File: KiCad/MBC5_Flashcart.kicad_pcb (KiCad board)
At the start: 2 copper layers, 51.1 x 61.3 mm, 10 parts, among them J0 CartBus, U1 MBC5, U2 MBM29F033C, U3 FM18W08

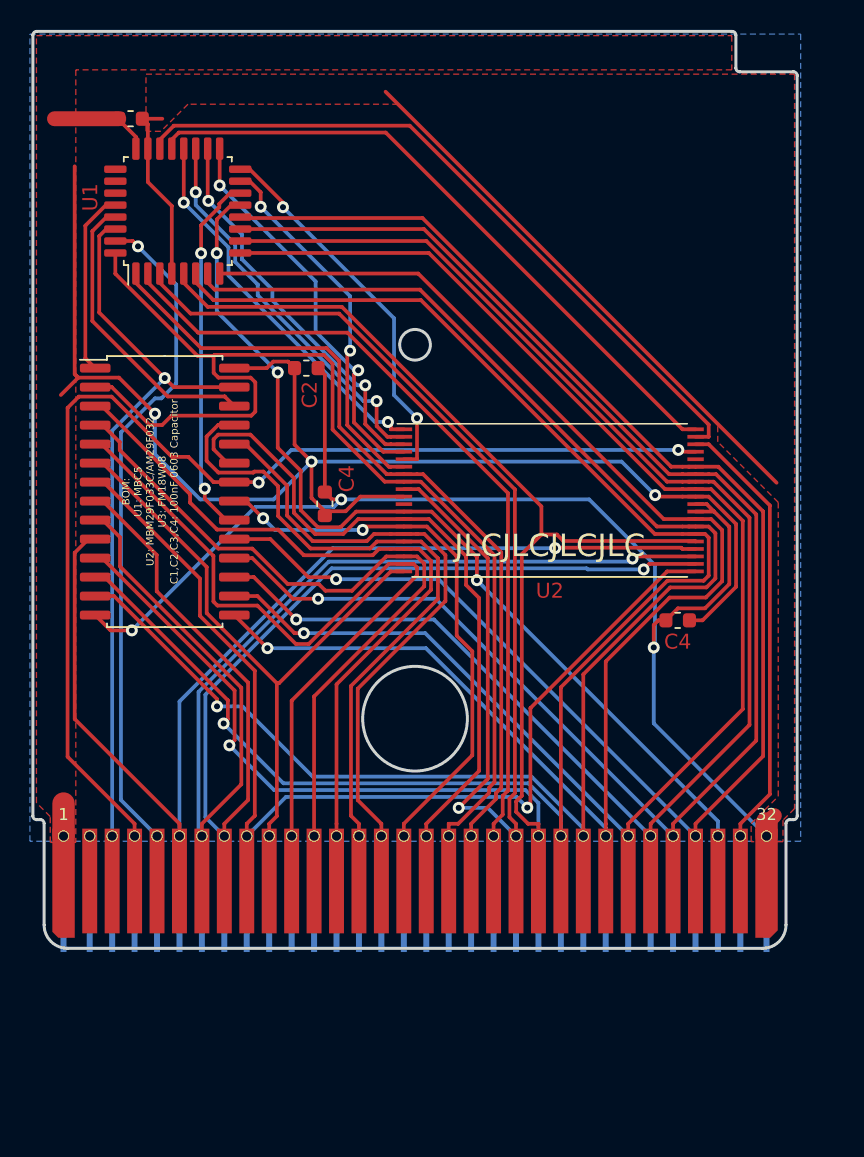
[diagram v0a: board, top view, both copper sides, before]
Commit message: Update to V2
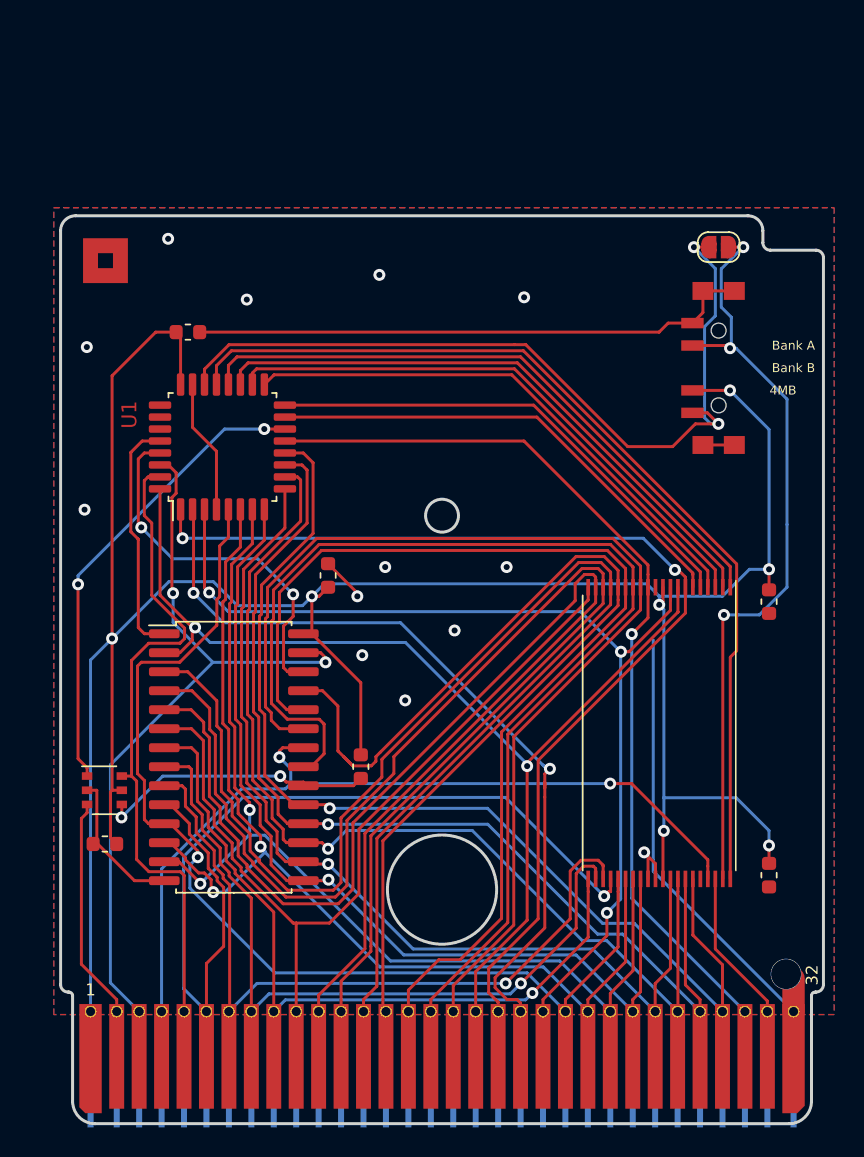
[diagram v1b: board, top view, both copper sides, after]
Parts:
- removed ? (x2): , 
- added C5: 100nF, Capacitor_SMD:C_0603_1608Metric, F.Cu at (120.1, 111.3)
- added H1: 3x3 Ground Pad, Custom:Nintendo_3x3_GNDPad, F.Cu at (120.1, 72.3)
- added JP1: Jumper_NO_Small, Jumper:SolderJumper-2_P1.3mm_Open_RoundedPad1.0x1.5mm, F.Cu at (161.1, 71.4)
- added PAD*: GBA-ProductionIndicator, Custom:GBA-ProductionIndicator, B.Cu at (156.7, 77.9)
- added R1: 10K, Resistor_SMD:R_0603_1608Metric, F.Cu at (137.2, 106.1)
- added ROM Mode: SW_SP3T, Custom:CUS-13TB-Aliex SP3T, F.Cu at (161.1, 79.5)
- added U4: 74LVC1G332GW,125, Package_SO:TSOP-6_1.65x3.05mm_P0.95mm, F.Cu at (120.0, 107.7)
- moved C4 30.4 mm to (164.5, 95.1), turned to -90 degrees
- moved U2 18.5 mm to (158.1, 103.9), turned to -90 degrees
- moved U3 18.3 mm to (128.7, 105.5)
- moved C3 18.1 mm to (164.5, 113.4), turned to -90 degrees
- moved U1 16.1 mm to (127.9, 84.8)
- moved C1 14.8 mm to (125.6, 77.1)
- moved C2 13.9 mm to (135.0, 93.3), turned to 90 degrees
- moved J0 11.9 mm to (142.6, 130.0)
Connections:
- U1 pad 22: RA21 -> RA21_MBC
- U1 pad 25: Net-(U1-Pad25) -> unconnected-(U1-Pad25)
- U1 pad 26: Net-(U1-Pad26) -> unconnected-(U1-Pad26)
- U1 pad 27: Net-(U1-Pad27) -> unconnected-(U1-Pad27)
- U2 pad 11: Net-(U2-Pad11) -> unconnected-(U2-Pad11)
- U2 pad 36: Net-(U2-Pad36) -> unconnected-(U2-Pad36)
- U3 pad 20: RAMCS -> #CE
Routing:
- net +5V: track 105.8 -> 175.9 mm, vias 3 -> 7
- net RA21_MBC: track 0.00 -> 56.0 mm, vias 0 -> 2
- net GND: track 141.0 -> 99.0 mm, vias 3 -> 14
- net A7: track 48.4 -> 89.3 mm
- net A6: track 49.3 -> 88.4 mm
- net A10: track 37.6 -> 76.7 mm, vias 2 -> 0
- net D1: track 107.8 -> 70.2 mm, vias 1 -> 2
- net D2: track 106.7 -> 69.1 mm, vias 1 -> 2
- net D0: track 106.3 -> 70.9 mm
- net A5: track 52.6 -> 87.4 mm
- net D7: track 105.7 -> 71.5 mm
- net D3: track 97.1 -> 62.9 mm
- net D6: track 103.2 -> 69.7 mm
- net D4: track 98.3 -> 65.5 mm
- net D5: track 100.7 -> 68.6 mm
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- removed copper zone on F.Cu, net +5V
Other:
- board size 51.1 x 61.3 mm -> 51 x 60.7 mm
- net class Default removed
- rule pad_to_mask_clearance: 0.05 -> 0
- board text added: "'22"
- board text added: "1"
- board text added: "12"
- board text added: "4MB"
- board text added: "6"
- board text added: "7"
- board text added: "Bank A"
- board text added: "Bank B"
- board text removed: "BOM: U1: MBC5 U2: MBM29F033C/AM29F032 U3: FM18W08 C1,C2,C3,C4: 100nF 0603 Capacitor"
- board text removed: "C1"
- board text removed: "C2"
- board text removed: "C4"
- board text removed: "JLCJLCJLCJLC"
- board text removed: "U1"
- board text removed: "U2"
- board text removed: "U3"

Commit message: Release V3
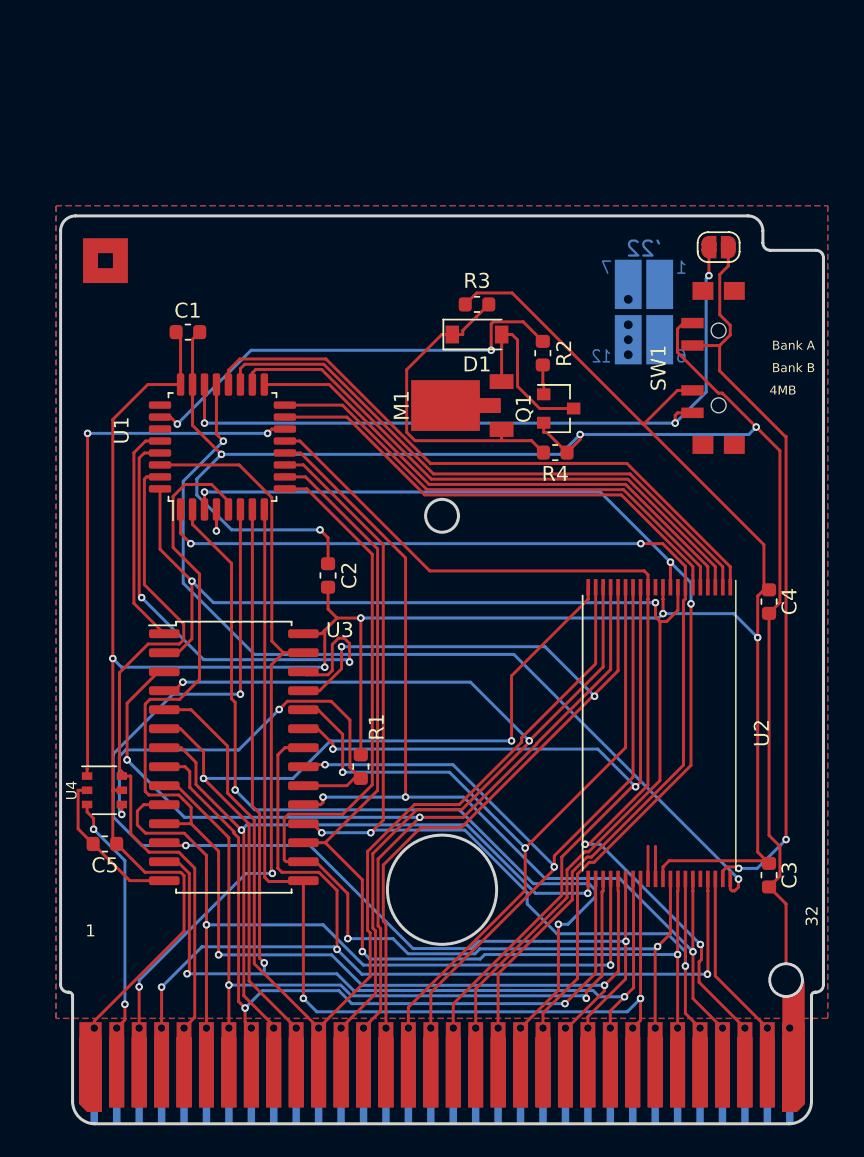
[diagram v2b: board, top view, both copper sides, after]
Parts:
- removed PAD*: GBA-ProductionIndicator, Custom:GBA-ProductionIndicator
- added A**: June, HDR_Gameboy_Date_Indicators:08 August, B.Cu at (156.1, 75.7)
- added D1: D, Diode_SMD:D_SOD-123, F.Cu at (145.0, 77.2)
- added M1: Motor_DC, Custom:ANDA-T1035, F.Cu at (144.0, 82.0)
- added Q1: BC817-40,215, Package_TO_SOT_SMD:SOT-23, F.Cu at (150.4, 82.2)
- added R2: 30K, Resistor_SMD:R_0603_1608Metric, F.Cu at (149.4, 78.5)
- added R3: 15Ω, Resistor_SMD:R_0603_1608Metric, F.Cu at (145.0, 75.2)
- added R4: 22Ω, Resistor_SMD:R_0603_1608Metric, F.Cu at (150.2, 85.1)
- J0: footprint Connector_GameBoy:GameBoy_GamePak_CGB-002_P1.50mm_Edge -> HDR_Gameboy_Cartridges:GB_Cartridge
- SW1: renamed from ROM Mode
- moved J0 3.94 mm to (142.6, 126.1)
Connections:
- SW1 pad 0: GND -> (no net)
- U1 pad 26: unconnected-(U1-Pad26) -> Rumble
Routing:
- net GND: track 99.0 -> 139.1 mm, vias 14 -> 6
- net Rumble: track 0.00 -> 30.2 mm, vias 0 -> 2
- net Net-(D1-Pad1): track 0.00 -> 22.1 mm
- net A6: track 88.4 -> 67.9 mm, vias 0 -> 2
- net A7: track 89.3 -> 69.4 mm, vias 0 -> 2
- net A10: track 76.7 -> 57.7 mm, vias 0 -> 2
- net A5: track 87.4 -> 68.6 mm
- net D2: track 69.1 -> 83.6 mm, vias 2 -> 3
- net D0: track 70.9 -> 85.2 mm, vias 1 -> 2
- net RD: track 56.0 -> 68.5 mm, vias 2 -> 3
- net A9: track 70.5 -> 58.6 mm, vias 0 -> 2
- net Net-(D1-Pad2): track 0.00 -> 11.8 mm
- net A11: track 73.5 -> 61.8 mm, vias 0 -> 2
- net #CE: track 18.6 -> 30.3 mm
- net A12: track 73.5 -> 84.5 mm
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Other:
- outline, holes or cut-outs redrawn
- board text removed: "'22"
- board text removed: "1"
- board text removed: "12"
- board text removed: "6"
- board text removed: "7"
